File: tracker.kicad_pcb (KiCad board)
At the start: 2 copper layers, 50 x 37 mm, 43 parts, among them J2 Tag connect, J6 BATT, U1 MCP73831-2-OT, U2 W25X40CL, U3 STM32L432KBUx, U4 TPS78233DDC, U5 SIM808, Y1 32.768KHz

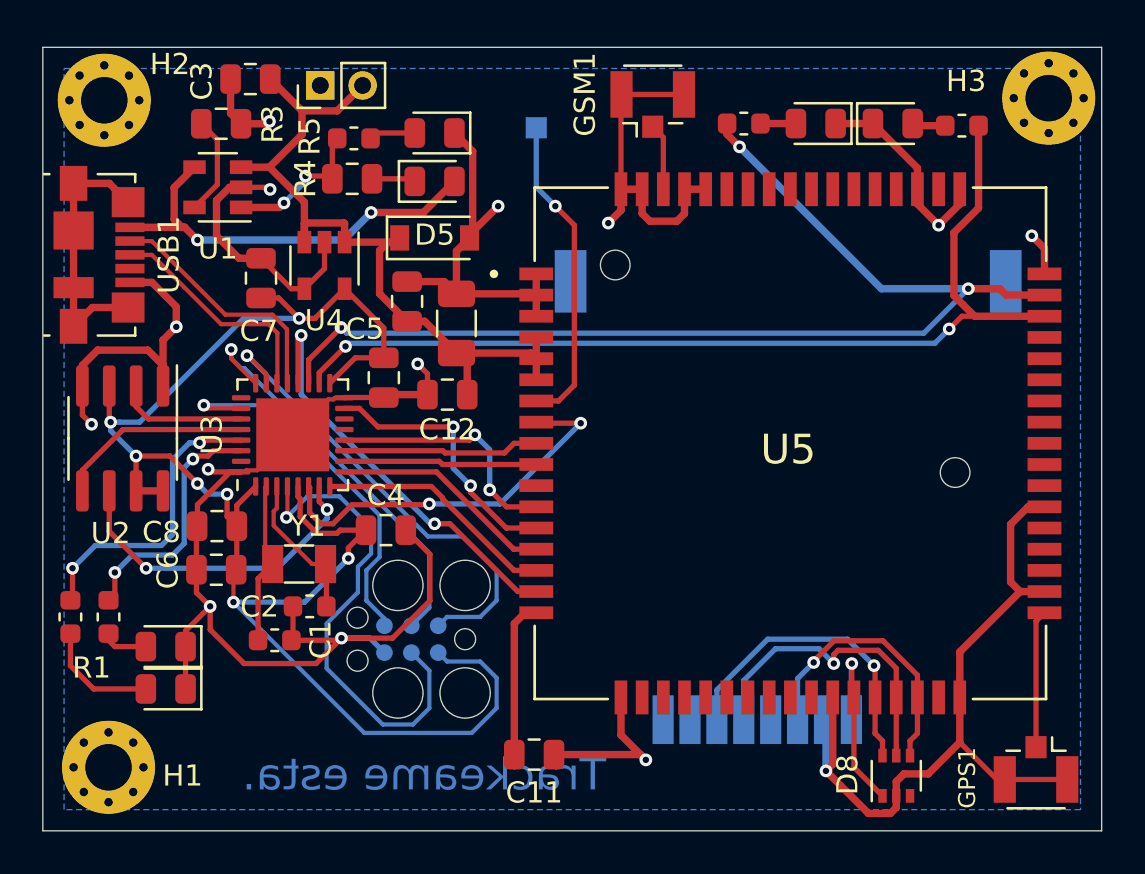
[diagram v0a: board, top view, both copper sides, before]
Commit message: Size reduction
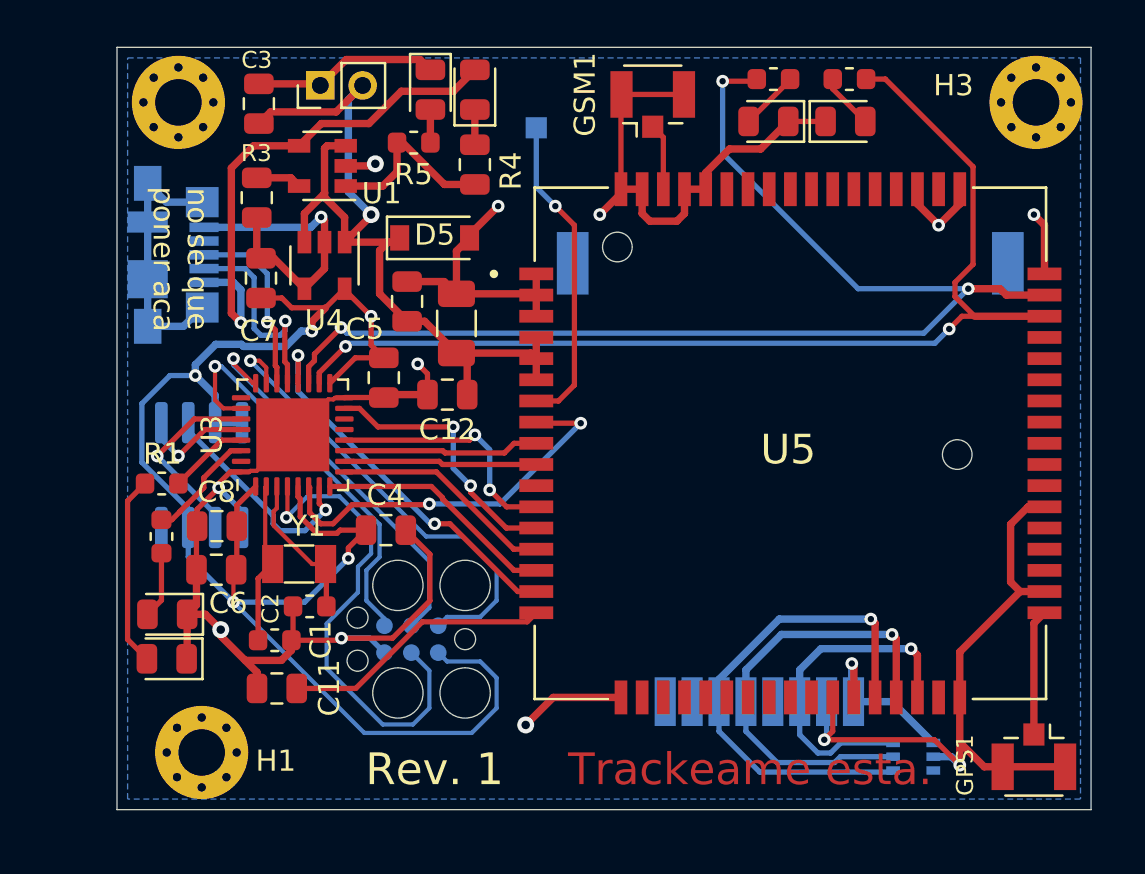
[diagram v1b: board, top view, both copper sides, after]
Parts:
- D8, U2, USB1: moved to B.Cu
- moved C11 12.5 mm to (167.1, 140.3), turned to 180 degrees
- moved R1 7.63 mm to (161.6, 130.6), turned to 0 degrees
- moved R4 5.83 mm to (176.4, 115.5), turned to 270 degrees
- moved R7 5.75 mm to (194.1, 111.5)
- moved U1 5.04 mm to (169.2, 115.6)
- moved D3 4.73 mm to (176.4, 112.0), turned to 90 degrees
- moved R2 4.55 mm to (161.6, 133.1)
- moved H1 4.46 mm to (163.5, 143.3)
- moved U2 4.11 mm to (163.5, 130.2), turned to 90 degrees
- moved R3 3.87 mm to (166.1, 117.1), turned to 90 degrees
- moved H2 3.50 mm to (162.4, 112.6)
- moved USB1 3.50 mm to (162.2, 119.8), turned to 90 degrees
- moved R5 2.83 mm to (173.5, 114.5)
- moved R6 2.52 mm to (190.5, 111.5)
- moved D6 2.24 mm to (190.3, 113.5)
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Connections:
- D8 pad 4: SIM_RST -> SIM_DATA
- D8 pad 6: SIM_DATA -> SIM_RST
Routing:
- net GND: track 170.6 -> 154.6 mm, vias 14 -> 13
- net /LED2: track 14.1 -> 3.81 mm, vias 2 -> 0
- net SIM_DATA: track 14.7 -> 23.6 mm
- net /LED1: track 11.9 -> 5.40 mm, vias 2 -> 0
- net SIM_CLK: track 14.9 -> 21.2 mm
- net Net-(C11-Pad1): track 7.44 -> 12.8 mm
- net VDD: track 36.1 -> 41.0 mm, vias 0 -> 1
- net /SPI1_SCK: track 15.6 -> 10.7 mm, vias 2 -> 1
- net STATUS: track 45.7 -> 50.4 mm
- net NETLIGHT: track 52.5 -> 56.9 mm
- net +5V: track 20.2 -> 24.4 mm, vias 2 -> 1
- net /SPI1_MOSI: track 9.27 -> 5.39 mm, vias 0 -> 1
- net Net-(D1-Pad2): track 5.53 -> 8.99 mm
- net SIM_RST: track 13.0 -> 16.1 mm
- net /SPI1_MISO: track 6.17 -> 9.20 mm, vias 0 -> 1
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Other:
- board size 50 x 37 mm -> 46 x 36 mm
- board text added: "no se que poner aca"
